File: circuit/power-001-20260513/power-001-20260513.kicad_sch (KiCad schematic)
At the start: 57 parts, among them J1 VIN, J2 +5V_{Line}, J3 Power, J4 Logic, J5 Sub_{Power}, J6 Sub_{Signal}, Q1 BSS138, Q2 PMOS, SW1 SW_SPDT, SW2 SW_SPDT, SW3 SW_SPDT, SW4 Locker_SW, U1 OKL-T/6-W12N-C, U2 OKL-T/6-W12N-C, U3 AZ1084-3.3, U4 BP5293-33, U5 PIC12F683-xSN

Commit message: Update コートヤード要件を追加した
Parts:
- F1: footprint (none) -> @Thrive_footprint_power:MF61NR_FUC-04
- SW4: footprint (none) -> @Thrive_footprint_power:DS-850K-S-ON-K
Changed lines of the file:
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@@
 			)
 		)
-		(property "Footprint" ""
+		(property "Footprint" "@Thrive_footprint_power:MF61NR_FUC-04"
 			(at 34.29 32.258 90)
 			(hide yes)
@@
 			)
 		)
-		(property "Footprint" ""
+		(property "Footprint" "@Thrive_footprint_power:DS-850K-S-ON-K"
 			(at 45.72 30.48 0)
 			(hide yes)

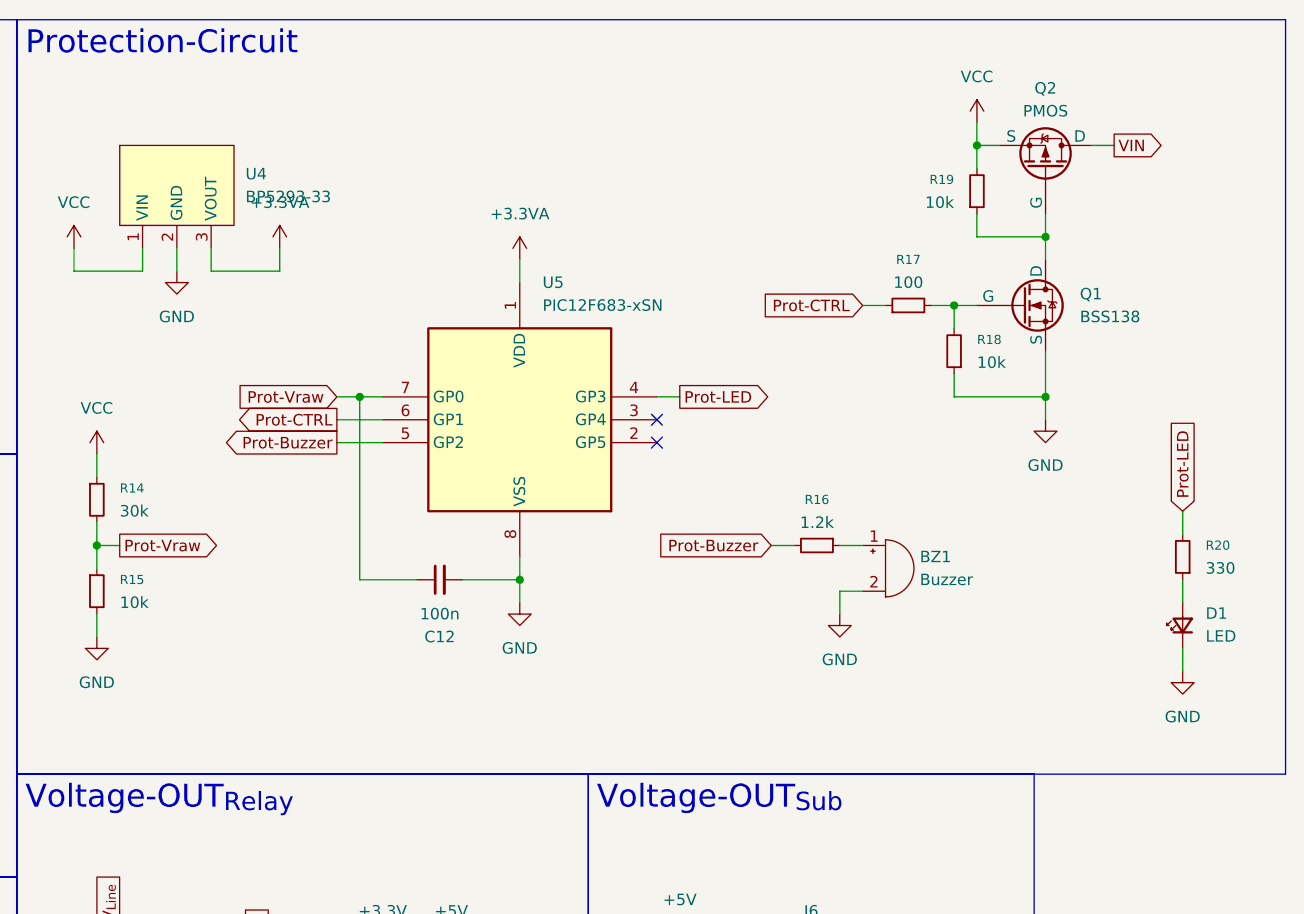
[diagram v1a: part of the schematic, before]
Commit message: Update ちょっと電源基板を修正
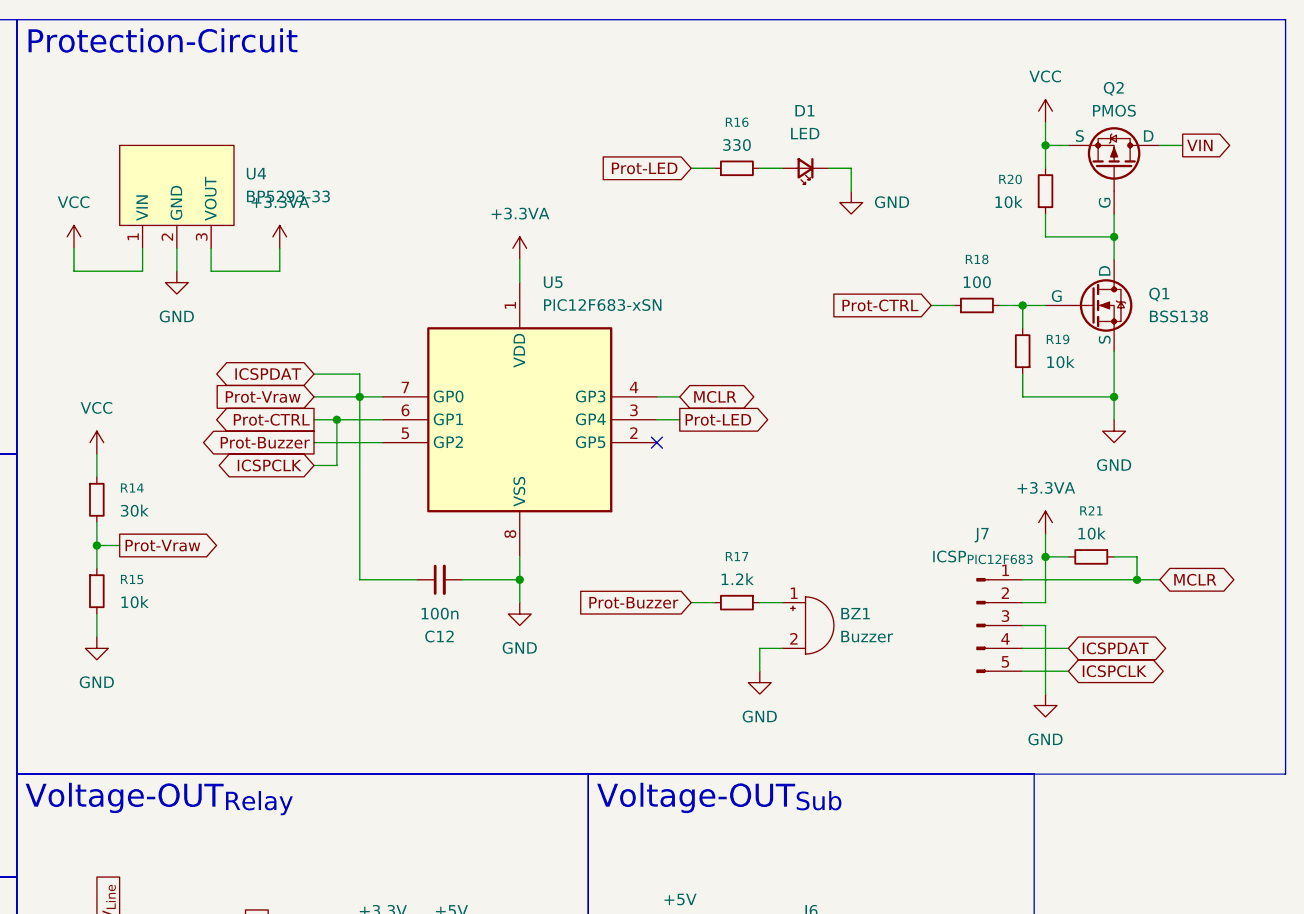
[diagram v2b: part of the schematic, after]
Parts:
- removed R20: 330, Resistor_SMD:R_0805_2012Metric, symbol Device:R_Small
- added J7: ICSP_{PIC12F683}, Connector_PinHeader_2.54mm:PinHeader_1x05_P2.54mm_Vertical, symbol Connector:Conn_01x05_Pin
- added R16: 330, Resistor_SMD:R_0805_2012Metric, symbol Device:R_Small
- added R21: 10k, Resistor_SMD:R_0805_2012Metric, symbol Device:R_Small
- D1: footprint Capacitor_SMD:C_0603_1608Metric -> LED_SMD:LED_0603_1608Metric
- renumbered R16 to R17, R17 to R18, R18 to R19, R19 to R20
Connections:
- net +3.3VA: now also J7.2 (Pin_2), R21.2
- net GND: now also J7.3 (Pin_3)
- net Prot-LED: now also U5.3 (GP4), R16.1; no longer U5.4 (GP3)
- net at D1.2 (A): now also R16.2
- net Prot-CTRL renamed ICSPCLK
- net ICSPCLK: now also J7.5 (Pin_5)
- net Prot-Vraw renamed ICSPDAT
- net ICSPDAT: now also J7.4 (Pin_4)
- new net MCLR: J7.1 (Pin_1), R21.1, U5.4 (GP3)
- no-connect marks 2 -> 1
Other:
- moved on the sheet: BZ1, Q1, Q2, R17, R18, R19, R20

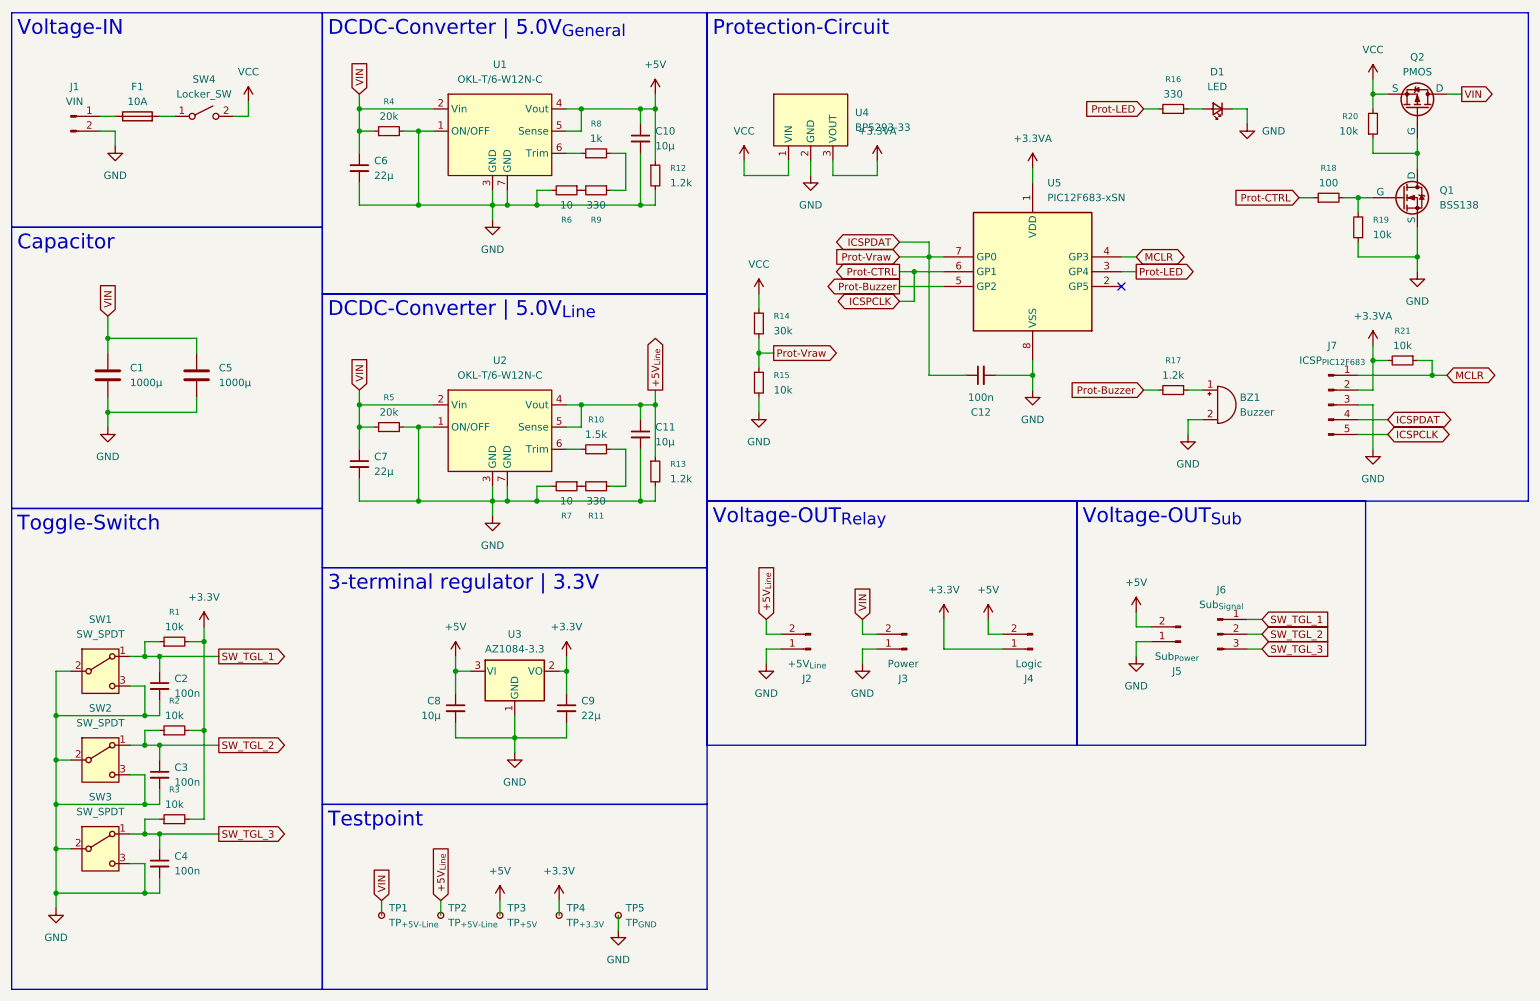
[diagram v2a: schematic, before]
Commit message: Update 電源基板の配置が苦しい
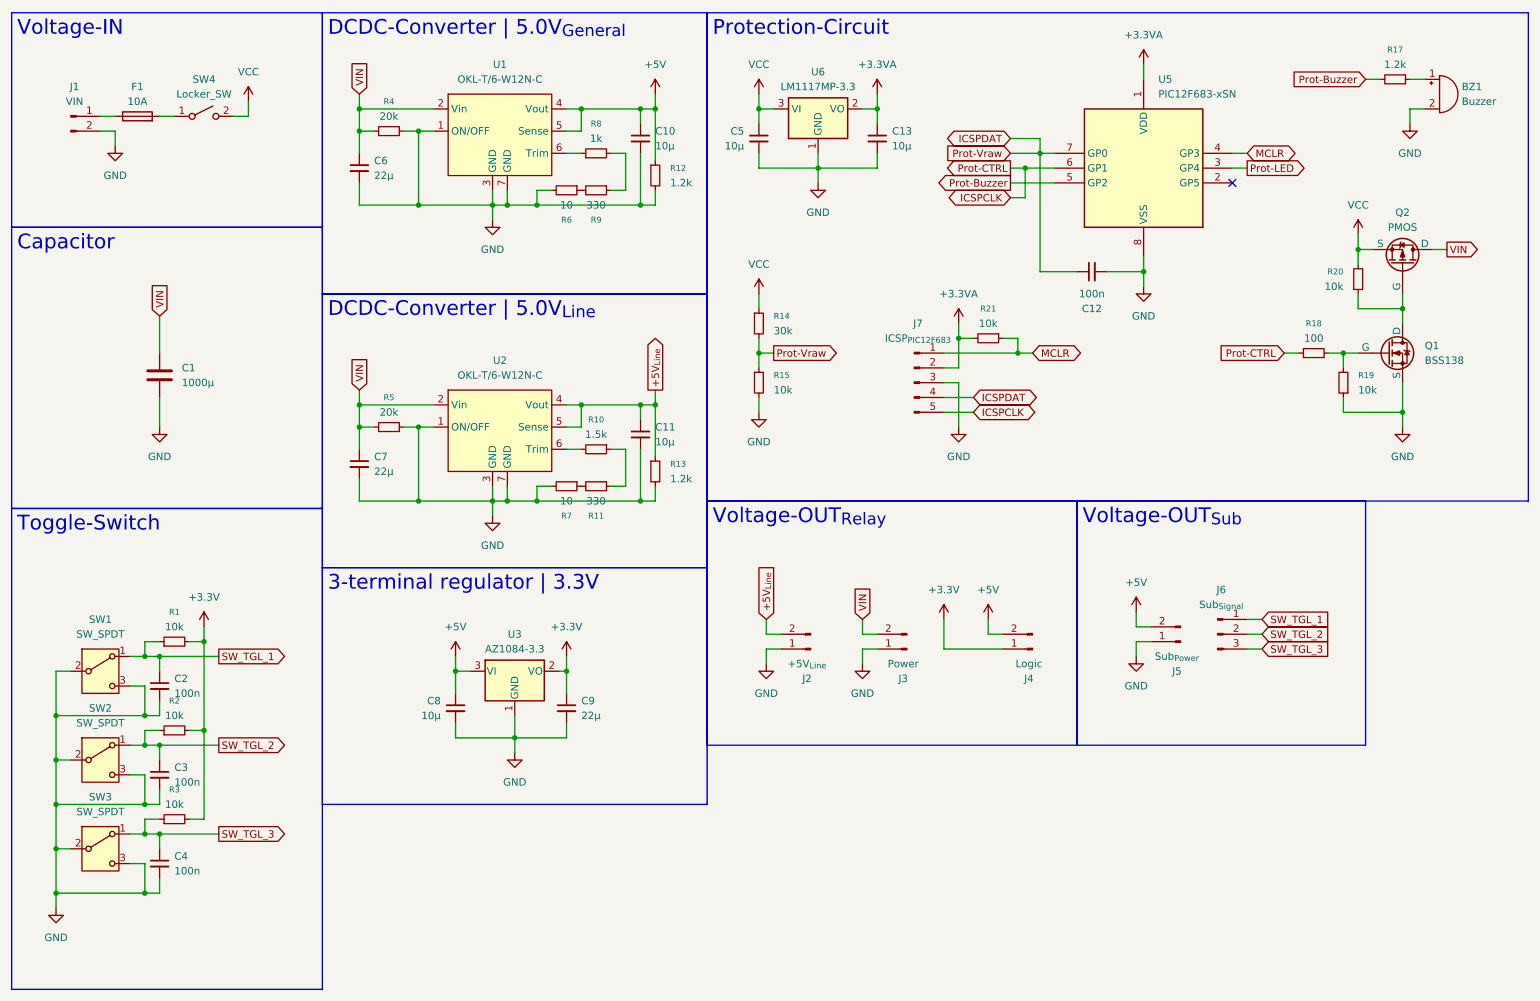
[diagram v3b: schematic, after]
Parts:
- removed C5: 1000μ, Capacitor_THT:CP_Radial_D10.0mm_P5.00mm, symbol Device:C
- removed D1: LED, LED_SMD:LED_0603_1608Metric, symbol Device:LED_Small
- removed R16: 330, Resistor_SMD:R_0805_2012Metric, symbol Device:R_Small
- removed TP1, TP2: TP_{+5V-Line}, TestPoint:TestPoint_Loop_D1.80mm_Drill1.0mm_Beaded, symbol Connector:TestPoint_Small
- removed TP3: TP_{+5V}, TestPoint:TestPoint_Loop_D1.80mm_Drill1.0mm_Beaded, symbol Connector:TestPoint_Small
- removed TP4: TP_{+3.3V}, TestPoint:TestPoint_Loop_D1.80mm_Drill1.0mm_Beaded, symbol Connector:TestPoint_Small
- removed TP5: TP_{GND}, TestPoint:TestPoint_Loop_D1.80mm_Drill1.0mm_Beaded, symbol Connector:TestPoint_Small
- removed U4: BP5293-33, @Thrive_footprint_power:BP5293-33, symbol @Thrive_symbol_power:BP5293-33
- added C13, C5: 10μ, Capacitor_SMD:C_0805_2012Metric, symbol Device:C_Small
- added U6: LM1117MP-3.3, Package_TO_SOT_SMD:SOT-223-3_TabPin2, symbol Regulator_Linear:LM1117MP-3.3
- J2, J3, J4, J5: footprint Connector_AMASS:AMASS_XT30PW-F_1x02_P2.50mm_Horizontal -> @Thrive_footprint_power:AMASS_XT30PW-F_1x02_P2.50mm_Horizontal
- J7: footprint Connector_PinHeader_2.54mm:PinHeader_1x05_P2.54mm_Vertical -> Connector_PinHeader_1.00mm:PinHeader_1x05_P1.00mm_Vertical
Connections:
- net +3.3VA: now also C13.1, U6.2 (VO)
- net GND: now also C13.2, C5.2, U6.1 (GND)
- net VCC: now also C5.1, U6.3 (VI)
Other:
- moved on the sheet: BZ1, C1, C12, J7, Q1, Q2, R17, R18, R19, R20, R21, U5
